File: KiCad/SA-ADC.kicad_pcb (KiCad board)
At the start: 4 copper layers, 99.1 x 94.2 mm, 226 parts, among them J1 Conn_01x03, J2 Conn_01x02, J3 Conn_01x08, SW1 SW_Push_SPDT, SW2 SW_Push, U1 40193, U10 74LVC1G32, U11 74LVC1G32, U12 74LVC1G32, U13 74LS21, U14 74LS21, U15 74LS21, U16 74LS21, U17 74LS21, U18 74AHC1G08, U19 74AHC1G08, U2 40193, U20 74LS21, U21 74AHC1G08, U22 74AHC1G08, U23 74LS21, U24 74LS21, U25 74AHC1G08, U26 74AHC1G08, U27 74AHC1G08, U28 74AHC1G08, U29 74LS21, U3 74HC04, U30 74LS21, U31 74AHC1G08, U32 74AHC1G08, U33 74AHC1G08, U34 LM358, U35 74LVC1G125, U36 74HC74, U37 LM317L_TO92, U38 L7805, U39 74HC74, U4 40245, U40 74HC74, U41 74HC74, U42 74LVC1G14, U43 74LS574, U44 LM555, U45 74LVC1G125, U46 74AHC1G08, U47 74LVC1G32, U48 74LVC1G125, U5 74LVC1G32, U6 74LVC1G32, U7 74LVC1G32, U8 74LVC1G32, U9 74LVC1G32

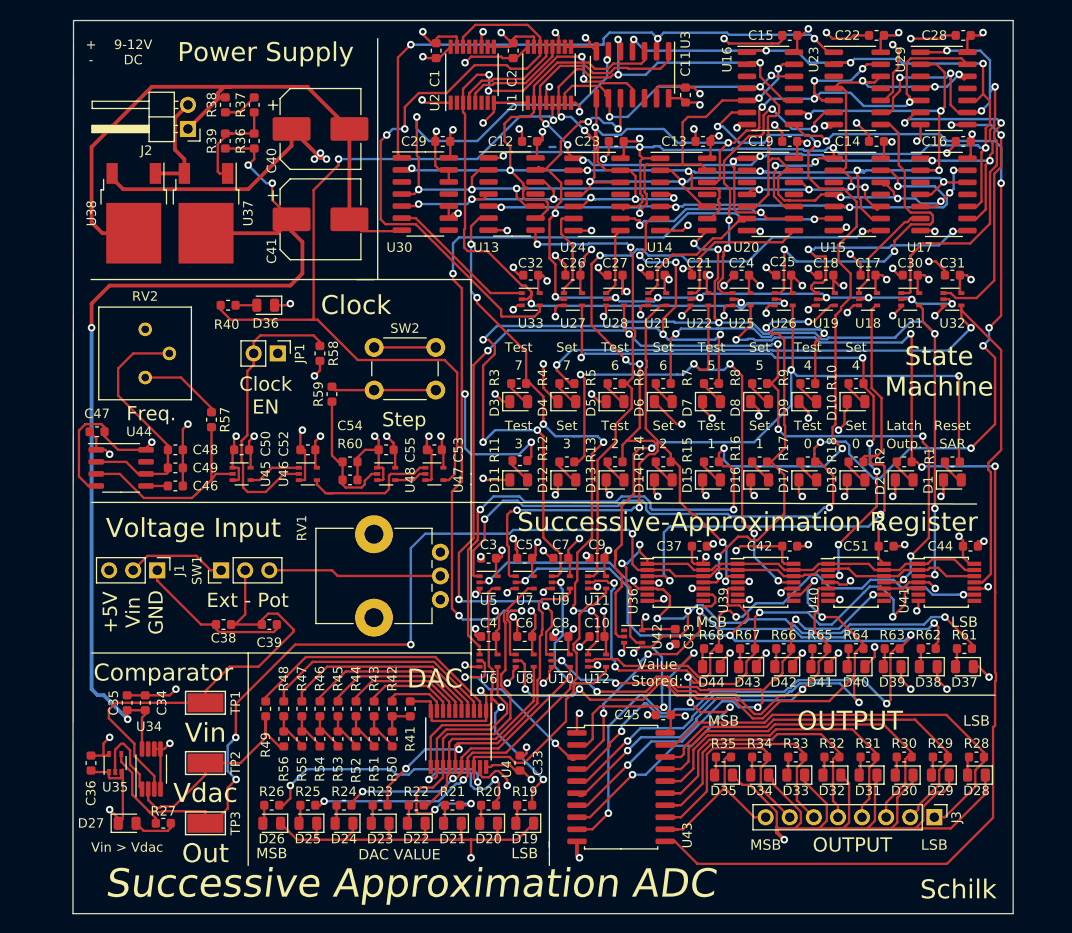
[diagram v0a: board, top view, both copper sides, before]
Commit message: First part placement
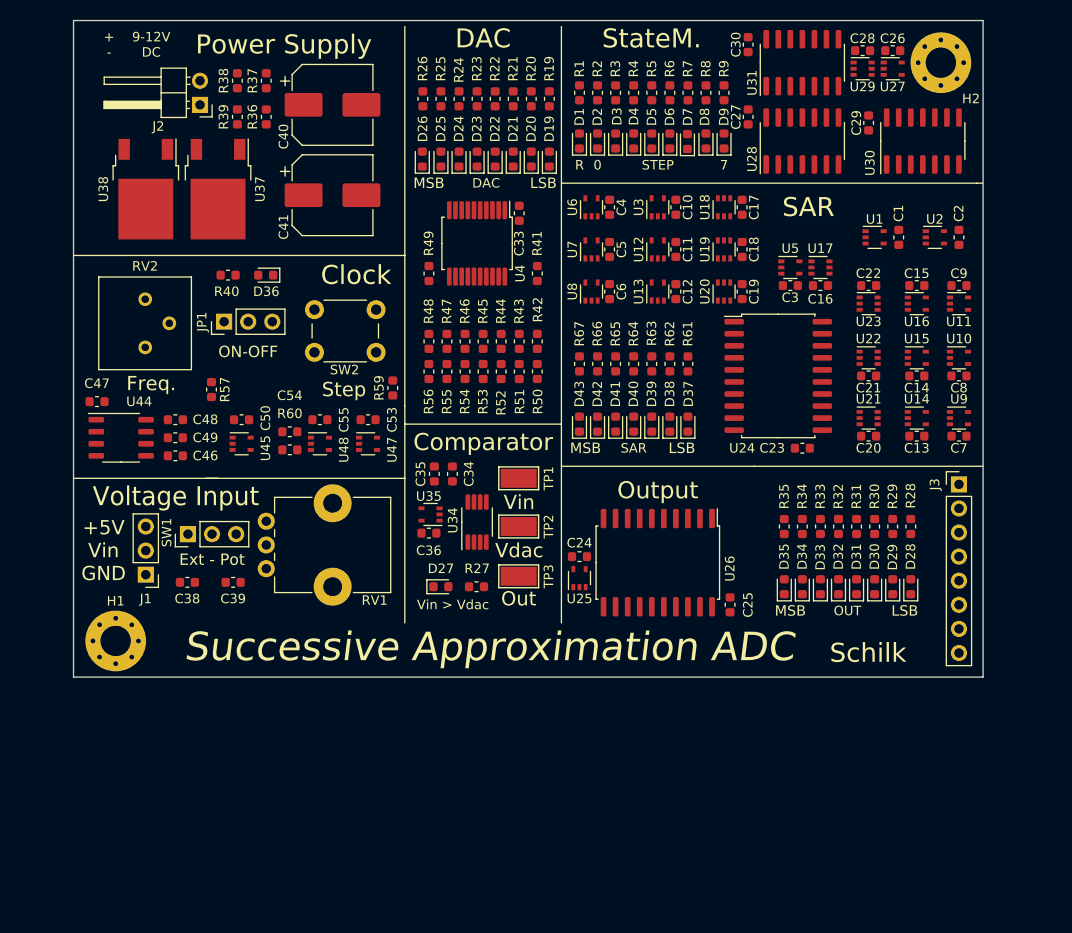
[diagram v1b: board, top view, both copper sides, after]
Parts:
- removed C31, C32, C37, C42, C43, C44, C45, C51, C52: 0u1, Capacitor_SMD:C_0603_1608Metric
- removed D10, D11, D12, D13, D14, D15, D16, D17, D18, D44: LED_Small, LED_SMD:LED_0805_2012Metric
- removed R10, R11, R12, R13, R14, R15, R16, R17, R18, R68: rled, Resistor_SMD:R_0603_1608Metric
- removed R58: 10K, Resistor_SMD:R_0603_1608Metric
- removed U32, U33, U46: 74AHC1G08, Package_TO_SOT_SMD:SOT-353_SC-70-5
- removed U36, U39, U40, U41: 74HC74, Package_SO:TSSOP-14_4.4x5mm_P0.65mm
- removed U42: 74LVC1G14, Package_TO_SOT_SMD:SOT-353_SC-70-5
- removed U43: 74LS574, Package_SO:SOIC-20W_7.5x12.8mm_P1.27mm
- added H1: MountingHole, MountingHole:MountingHole_3.2mm_M3_Pad_Via, F.Cu at (99.1, 111.8)
- added H2: MountingHole, MountingHole:MountingHole_3.2mm_M3_Pad_Via, F.Cu at (186.1, 50.8)
- D1, D19, D2, D20, D21, D22, D23, D24, D25, D26, D27, D28, D29, D3, D30, D31, D32, D33, D34, D35, D36, D37, D38, D39, D4, D40, D41, D42, D43, D5, D6, D7, D8, D9: footprint LED_SMD:LED_0805_2012Metric -> LED_SMD:LED_0603_1608Metric
- JP1: value Jumper_NC_Small -> Conn_01x03; footprint Connector_PinHeader_2.54mm:PinHeader_1x02_P2.54mm_Vertical -> Connector_PinHeader_2.54mm:PinHeader_1x03_P2.54mm_Vertical
- U1: value 40193 -> 74LVC1G04; footprint Package_SO:TSSOP-16_4.4x5mm_P0.65mm -> Package_TO_SOT_SMD:SOT-353_SC-70-5
- U13, U14, U15, U16: value 74LS21 -> 74LVC1G32; footprint Package_SO:SOIC-14_3.9x8.7mm_P1.27mm -> Package_TO_SOT_SMD:SOT-353_SC-70-5
- U17, U20, U23: value 74LS21 -> 74LVC1G157; footprint Package_SO:SOIC-14_3.9x8.7mm_P1.27mm -> Package_TO_SOT_SMD:SOT-363_SC-70-6
- U18, U19, U21, U22: value 74AHC1G08 -> 74LVC1G157; footprint Package_TO_SOT_SMD:SOT-353_SC-70-5 -> Package_TO_SOT_SMD:SOT-363_SC-70-6
- U2: value 40193 -> 74LVC1G08; footprint Package_SO:TSSOP-16_4.4x5mm_P0.65mm -> Package_TO_SOT_SMD:SOT-353_SC-70-5
- U24: value 74LS21 -> 74LS377; footprint Package_SO:SOIC-14_3.9x8.7mm_P1.27mm -> Package_SO:SOIC-20W_7.5x12.8mm_P1.27mm
- U25, U27: value 74AHC1G08 -> 74LVC1G04
- U26: value 74AHC1G08 -> 74LS377; footprint Package_TO_SOT_SMD:SOT-353_SC-70-5 -> Package_SO:SOIC-20W_7.5x12.8mm_P1.27mm
- U28: value 74AHC1G08 -> 74HC164; footprint Package_TO_SOT_SMD:SOT-353_SC-70-5 -> Package_SO:SOIC-14_3.9x8.7mm_P1.27mm
- U29: value 74LS21 -> 74LVC1G175; footprint Package_SO:SOIC-14_3.9x8.7mm_P1.27mm -> Package_TO_SOT_SMD:SOT-363_SC-70-6
- U3: value 74HC04 -> 74LVC1G32; footprint Package_SO:SOIC-14_3.9x8.7mm_P1.27mm -> Package_TO_SOT_SMD:SOT-353_SC-70-5
- U30: value 74LS21 -> 74HC02
- U31: value 74AHC1G08 -> 74HC02; footprint Package_TO_SOT_SMD:SOT-353_SC-70-5 -> Package_SO:SOIC-14_3.9x8.7mm_P1.27mm
- U4: value 40245 -> 74HC245; footprint Package_SO:TSSOP-20_4.4x6.5mm_P0.65mm -> Package_SO:SSOP-20_5.3x7.2mm_P0.65mm
- moved R26 76.2 mm to (131.4, 54.6), turned to 90 degrees
- moved R25 75.8 mm to (133.3, 54.6), turned to 90 degrees
- moved R24 75.4 mm to (135.3, 54.6), turned to 90 degrees
- moved R23 75.2 mm to (137.2, 54.6), turned to 90 degrees
- moved R22 74.9 mm to (139.1, 54.6), turned to 90 degrees
- moved R21 74.7 mm to (141.0, 54.6), turned to 90 degrees
- moved R20 74.6 mm to (142.9, 54.6), turned to 90 degrees
- moved R19 74.5 mm to (144.8, 54.6), turned to 90 degrees
- moved D26 71.8 mm to (131.4, 61.0), turned to 90 degrees
- moved D25 71.4 mm to (133.3, 61.0), turned to 90 degrees
- moved D24 71.1 mm to (135.3, 61.0), turned to 90 degrees
- moved D23 70.8 mm to (137.2, 61.0), turned to 90 degrees
- moved D22 70.5 mm to (139.1, 61.0), turned to 90 degrees
- moved D21 70.3 mm to (141.0, 61.0), turned to 90 degrees
- moved D20 70.2 mm to (142.9, 61.0), turned to 90 degrees
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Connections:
- C17 pad 1: +5V -> GND
- C17 pad 2: GND -> +5V
- C18 pad 1: +5V -> GND
- C18 pad 2: GND -> +5V
- C2 pad 1: +5V -> GND
- C2 pad 2: GND -> +5V
- C20 pad 1: +5V -> GND
- C20 pad 2: GND -> +5V
- C21 pad 1: +5V -> GND
- C21 pad 2: GND -> +5V
- C25 pad 1: +5V -> GND
- C25 pad 2: GND -> +5V
- C28 pad 1: GND -> +5V
- C28 pad 2: +5V -> GND
- C29 pad 1: GND -> +5V
- C29 pad 2: +5V -> GND
- JP1 pad 1: +5V -> Net-(JP1-Pad1)
- R1 pad 2: /SA-Register.sch/Reset -> /SA-Register.sch/STATE_RST
- R2 pad 2: /Output/LatchOutput -> /SA-Register.sch/STATE0
- R3 pad 2: /SA-Register.sch/Test7 -> /SA-Register.sch/STATE1
- R4 pad 2: /SA-Register.sch/Latch7 -> /SA-Register.sch/STATE2
- R5 pad 2: /SA-Register.sch/Test6 -> /SA-Register.sch/STATE3
- R6 pad 2: /SA-Register.sch/Latch6 -> /SA-Register.sch/STATE4
- R60 pad 1: Net-(C54-Pad1) -> Net-(R59-Pad2)
- R7 pad 2: /SA-Register.sch/Test5 -> /SA-Register.sch/STATE5
- R8 pad 2: /SA-Register.sch/Latch5 -> /SA-Register.sch/STATE6
- R9 pad 2: /SA-Register.sch/Test4 -> /Analog/D7
- U1 pad 1: GND -> (no net)
- U1 pad 2: /StateMaschine.sch/Counter/C1 -> /SA-Register.sch/STATE_RST
- U1 pad 3: /StateMaschine.sch/Counter/C0 -> GND
- U1 pad 4: +5V -> Net-(U1-Pad4)
- U1 pad 5: /Clock/CLK -> +5V
- U10 pad 1: /SA-Register.sch/Test5 -> /SA-Register.sch/STATE5
- U11 pad 1: /SA-Register.sch/Test6 -> /SA-Register.sch/STATE6
- U12 pad 1: /SA-Register.sch/Test7 -> /SA-Register.sch/STATE2
- U12 pad 2: /Output/OUT_7 -> /SA-Register.sch/STATE_RST
- U12 pad 4: /Analog/D7 -> Net-(U12-Pad4)
- U13 pad 1: /StateMaschine.sch/StateDecode/~1 -> /SA-Register.sch/STATE3
- U13 pad 2: /StateMaschine.sch/StateDecode/~2 -> /SA-Register.sch/STATE_RST
- U13 pad 3: (no net) -> GND
- U13 pad 4: /StateMaschine.sch/StateDecode/~3 -> Net-(U13-Pad4)
- U13 pad 5: /StateMaschine.sch/StateDecode/~4 -> +5V
- U14 pad 1: /StateMaschine.sch/StateDecode/~1 -> /SA-Register.sch/STATE4
- U14 pad 2: /StateMaschine.sch/Counter/C2 -> /SA-Register.sch/STATE_RST
- U14 pad 3: (no net) -> GND
- U14 pad 4: /StateMaschine.sch/StateDecode/~3 -> Net-(U14-Pad4)
- U14 pad 5: /StateMaschine.sch/StateDecode/~4 -> +5V
- U15 pad 1: /StateMaschine.sch/StateDecode/~1 -> /SA-Register.sch/STATE5
- U15 pad 2: /StateMaschine.sch/StateDecode/~2 -> /SA-Register.sch/STATE_RST
- U15 pad 3: (no net) -> GND
- U15 pad 4: /StateMaschine.sch/Counter/C3 -> Net-(U15-Pad4)
- U15 pad 5: /StateMaschine.sch/StateDecode/~4 -> +5V
- U16 pad 1: /StateMaschine.sch/StateDecode/~1 -> /SA-Register.sch/STATE6
- U16 pad 2: /StateMaschine.sch/Counter/C2 -> /SA-Register.sch/STATE_RST
- U16 pad 3: (no net) -> GND
- U16 pad 4: /StateMaschine.sch/Counter/C3 -> Net-(U16-Pad4)
- U16 pad 5: /StateMaschine.sch/StateDecode/~4 -> +5V
- U17 pad 1: /StateMaschine.sch/Counter/C0 -> /Analog/COMP_OUT
- U17 pad 2: /StateMaschine.sch/Counter/C1 -> GND
- U17 pad 3: (no net) -> /Output/OUT_0
- U17 pad 4: /StateMaschine.sch/Counter/C2 -> Net-(U17-Pad4)
- U17 pad 5: /StateMaschine.sch/Counter/C3 -> +5V
- U17 pad 6: Net-(U17-Pad6) -> /SA-Register.sch/STATE0
- U18 pad 1: Net-(U17-Pad6) -> /SA-Register.sch/D
- U18 pad 2: /StateMaschine.sch/StateDecode/~4 -> GND
- U18 pad 3: GND -> /Output/OUT_1
- U18 pad 4: /SA-Register.sch/Latch0 -> Net-(U18-Pad4)
- U19 pad 1: Net-(U17-Pad8) -> /SA-Register.sch/D
- U19 pad 2: /StateMaschine.sch/StateDecode/~4 -> GND
- U19 pad 3: GND -> /Output/OUT_2
- U19 pad 4: /SA-Register.sch/Latch1 -> Net-(U19-Pad4)
- U2 pad 1: GND -> Net-(U1-Pad4)
- U2 pad 2: Net-(U2-Pad2) -> /Analog/COMP_OUT
- U2 pad 3: /StateMaschine.sch/Counter/C4 -> GND
- U2 pad 4: Net-(U1-Pad13) -> /SA-Register.sch/D
- U2 pad 5: Net-(U1-Pad12) -> +5V
- U20 pad 1: /StateMaschine.sch/Counter/C0 -> /SA-Register.sch/D
- U20 pad 2: /StateMaschine.sch/Counter/C1 -> GND
- U20 pad 3: (no net) -> /Output/OUT_3
- U20 pad 4: /StateMaschine.sch/StateDecode/~2 -> Net-(U20-Pad4)
- U20 pad 5: /StateMaschine.sch/Counter/C3 -> +5V
- U20 pad 6: Net-(U20-Pad6) -> Net-(U13-Pad4)
- U21 pad 1: Net-(U20-Pad6) -> /SA-Register.sch/D
- U21 pad 2: /StateMaschine.sch/StateDecode/~4 -> GND
- U21 pad 3: GND -> /Output/OUT_4
- U21 pad 4: /SA-Register.sch/Latch2 -> Net-(U21-Pad4)
- U22 pad 1: Net-(U20-Pad8) -> /SA-Register.sch/D
- U22 pad 2: /StateMaschine.sch/StateDecode/~4 -> GND
- U22 pad 3: GND -> /Output/OUT_5
- U22 pad 4: /SA-Register.sch/Latch3 -> Net-(U22-Pad4)
- U23 pad 1: /StateMaschine.sch/StateDecode/~0 -> /SA-Register.sch/D
- U23 pad 2: /StateMaschine.sch/StateDecode/~1 -> GND
- U23 pad 3: (no net) -> /Output/OUT_6
- U23 pad 4: /StateMaschine.sch/StateDecode/~2 -> Net-(U23-Pad4)
- U23 pad 5: /StateMaschine.sch/StateDecode/~3 -> +5V
- U23 pad 6: Net-(U23-Pad6) -> Net-(U16-Pad4)
- U24 pad 1: /StateMaschine.sch/Counter/C0 -> GND
- U24 pad 10: /StateMaschine.sch/StateDecode/~1 -> GND
- U24 pad 11: (no net) -> /Clock/CLK
- U24 pad 12: /StateMaschine.sch/Counter/C2 -> /Output/OUT_4
- U24 pad 13: /StateMaschine.sch/StateDecode/~3 -> Net-(U21-Pad4)
- U24 pad 14: +5V -> Net-(U22-Pad4)
- U24 pad 2: /StateMaschine.sch/Counter/C1 -> /Output/OUT_0
- U24 pad 3: (no net) -> Net-(U17-Pad4)
- U24 pad 4: /StateMaschine.sch/Counter/C2 -> Net-(U18-Pad4)
- U24 pad 5: /StateMaschine.sch/StateDecode/~3 -> /Output/OUT_1
- U24 pad 6: Net-(U24-Pad6) -> /Output/OUT_2
- U24 pad 7: GND -> Net-(U19-Pad4)
- U24 pad 8: Net-(U24-Pad8) -> Net-(U20-Pad4)
- U24 pad 9: /StateMaschine.sch/Counter/C0 -> /Output/OUT_3
- U25 pad 1: Net-(U23-Pad6) -> (no net)
- U25 pad 2: /StateMaschine.sch/Counter/C4 -> /Analog/D7
- U25 pad 4: /Output/LatchOutput -> Net-(U25-Pad4)
- U26 pad 1: Net-(U23-Pad8) -> Net-(U25-Pad4)
- U26 pad 2: /StateMaschine.sch/Counter/C4 -> Net-(J3-Pad1)
- U26 pad 3: GND -> /Output/OUT_0
- U26 pad 4: /SA-Register.sch/Reset -> /Output/OUT_1
- U26 pad 5: +5V -> Net-(J3-Pad2)
- U27 pad 1: Net-(U24-Pad6) -> (no net)
- U27 pad 2: /StateMaschine.sch/StateDecode/~4 -> /Clock/CLK
- U27 pad 4: /SA-Register.sch/Latch4 -> Net-(U27-Pad4)
- U28 pad 1: Net-(U24-Pad8) -> /StateMaschine.sch/C_IN
- U28 pad 2: /StateMaschine.sch/StateDecode/~4 -> /StateMaschine.sch/C_IN
- U28 pad 3: GND -> /SA-Register.sch/STATE_RST
- U28 pad 4: /SA-Register.sch/Latch5 -> /SA-Register.sch/STATE0
- U28 pad 5: +5V -> /SA-Register.sch/STATE1
- U29 pad 1: /StateMaschine.sch/Counter/C0 -> Net-(U27-Pad4)
- U29 pad 2: /StateMaschine.sch/Counter/C1 -> GND
- U29 pad 3: (no net) -> /SA-Register.sch/STATE6
- U29 pad 4: /StateMaschine.sch/StateDecode/~2 -> /Analog/D7
- U29 pad 5: /StateMaschine.sch/StateDecode/~3 -> +5V
- U29 pad 6: Net-(U29-Pad6) -> +5V
- U3 pad 1: /StateMaschine.sch/Counter/C0 -> /SA-Register.sch/STATE1
- U3 pad 2: /StateMaschine.sch/StateDecode/~0 -> /SA-Register.sch/STATE_RST
- U3 pad 3: /StateMaschine.sch/Counter/C1 -> GND
- U3 pad 4: /StateMaschine.sch/StateDecode/~1 -> Net-(U18-Pad6)
- U3 pad 5: /StateMaschine.sch/Counter/C2 -> +5V
- U30 pad 1: /StateMaschine.sch/StateDecode/~0 -> Net-(U30-Pad1)
- U30 pad 10: GND -> Net-(U30-Pad10)
- U30 pad 11: (no net) -> /SA-Register.sch/STATE5
- U30 pad 12: GND -> /SA-Register.sch/STATE6
- U30 pad 13: GND -> Net-(U30-Pad13)
- U30 pad 2: /StateMaschine.sch/Counter/C1 -> /SA-Register.sch/STATE_RST
- U30 pad 3: (no net) -> /SA-Register.sch/STATE0
- U30 pad 4: /StateMaschine.sch/StateDecode/~2 -> Net-(U30-Pad4)
- U30 pad 5: /StateMaschine.sch/StateDecode/~3 -> /SA-Register.sch/STATE1
- U30 pad 6: Net-(U30-Pad6) -> /SA-Register.sch/STATE2
- U30 pad 8: Net-(U30-Pad8) -> /SA-Register.sch/STATE3
- U30 pad 9: GND -> /SA-Register.sch/STATE4
- U31 pad 1: Net-(U29-Pad6) -> Net-(U31-Pad1)
- U31 pad 2: /StateMaschine.sch/StateDecode/~4 -> Net-(U30-Pad1)
- U31 pad 3: GND -> Net-(U30-Pad4)
- U31 pad 4: /SA-Register.sch/Latch6 -> Net-(U31-Pad4)
- U31 pad 5: +5V -> Net-(U30-Pad10)
- U4 pad 1: GND -> +5V
- U4 pad 11: /Analog/D0 -> /Analog/DAC/D7
- U4 pad 12: /Analog/D1 -> /Analog/DAC/D6
- U4 pad 13: /Analog/D2 -> /Analog/DAC/D5
- U4 pad 14: /Analog/D3 -> /Analog/DAC/D4
- U4 pad 15: /Analog/D4 -> /Analog/DAC/D3
- U4 pad 16: /Analog/D5 -> /Analog/DAC/D2
- U4 pad 17: /Analog/D6 -> /Analog/DAC/D1
- U4 pad 18: /Analog/D7 -> /Analog/DAC/D0
- U4 pad 2: /Analog/DAC/D7 -> /Analog/D0
- U4 pad 3: /Analog/DAC/D6 -> /Analog/D1
- U4 pad 4: /Analog/DAC/D5 -> /Analog/D2
- U4 pad 5: /Analog/DAC/D4 -> /Analog/D3
- U4 pad 6: /Analog/DAC/D3 -> /Analog/D4
- U4 pad 7: /Analog/DAC/D2 -> /Analog/D5
- U4 pad 8: /Analog/DAC/D1 -> /Analog/D6
- U4 pad 9: /Analog/DAC/D0 -> /Analog/D7
- U45 pad 4: Net-(U45-Pad4) -> Net-(JP1-Pad1)
- U47 pad 1: Net-(U46-Pad4) -> Net-(JP1-Pad2)
- U5 pad 1: /SA-Register.sch/Test0 -> /SA-Register.sch/STATE0
- U6 pad 1: /SA-Register.sch/Test1 -> /SA-Register.sch/STATE1
- U7 pad 1: /SA-Register.sch/Test2 -> /SA-Register.sch/STATE2
- U8 pad 1: /SA-Register.sch/Test3 -> /SA-Register.sch/STATE3
- U9 pad 1: /SA-Register.sch/Test4 -> /SA-Register.sch/STATE4
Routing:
- net GND: track 513.6 -> 0.00 mm, vias 120 -> 0
- net +5V: track 259.7 -> 0.00 mm, vias 58 -> 0
- net /StateMaschine.sch/StateDecode/~4: track 179.4 -> 0.00 mm, vias 18 -> 0
- net /StateMaschine.sch/Counter/C0: track 150.9 -> 0.00 mm, vias 14 -> 0
- net /StateMaschine.sch/StateDecode/~1: track 149.8 -> 0.00 mm, vias 11 -> 0
- net /StateMaschine.sch/Counter/C1: track 144.6 -> 0.00 mm, vias 9 -> 0
- net /SA-Register.sch/Test0: track 131.3 -> 0.00 mm, vias 8 -> 0
- net /StateMaschine.sch/StateDecode/~2: track 130.9 -> 0.00 mm, vias 12 -> 0
- net /Analog/COMP_OUT: track 128.6 -> 0.00 mm, vias 4 -> 0
- net /StateMaschine.sch/StateDecode/~3: track 124.3 -> 0.00 mm, vias 13 -> 0
- net /SA-Register.sch/Test1: track 122.1 -> 0.00 mm, vias 6 -> 0
- net /Output/LatchOutput: track 121.1 -> 0.00 mm, vias 4 -> 0
- net /SA-Register.sch/Test3: track 112.0 -> 0.00 mm, vias 6 -> 0
- net VDDA: track 105.4 -> 0.00 mm, vias 4 -> 0
- net /Output/OUT_2: track 104.0 -> 0.00 mm, vias 5 -> 0
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- removed copper zone on In2.Cu, net +5V
- removed copper zone on In1.Cu, net GND
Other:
- board size 99.1 x 94.2 mm -> 95.9 x 69.2 mm
- board text added: "ON-OFF"
- board text added: "OUT"
- board text added: "Output"
- board text added: "R"
- board text added: "STEP"
- board text added: "StateM."
- board text removed: "1"
- board text removed: "2"
- board text removed: "3"
- board text removed: "4"
- board text removed: "5"
- board text removed: "6"
- board text removed: "Clock EN"
- board text removed: "DAC VALUE"
- board text removed: "Latch"
- board text removed: "OUTPUT"
- board text removed: "Outp."
- board text removed: "Reset"
- board text removed: "Set"
- board text removed: "State Machine"
- board text removed: "Successive-Approximation Register"
- board text removed: "Test"
- board text removed: "Value Stored:"
